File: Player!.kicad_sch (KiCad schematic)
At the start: 26 parts, among them J1 USB4085-GF-A_REVA4, J2 AVR-ISP-6, SW1 RotaryEncoder_Switch, SW2 SW_Push, SW3 SW_Push, SW4 SW_Push, SW5 SW_Push, SW6 Reset, SW7 Boot, U1 ATmega328P-P, Y1 Crystal

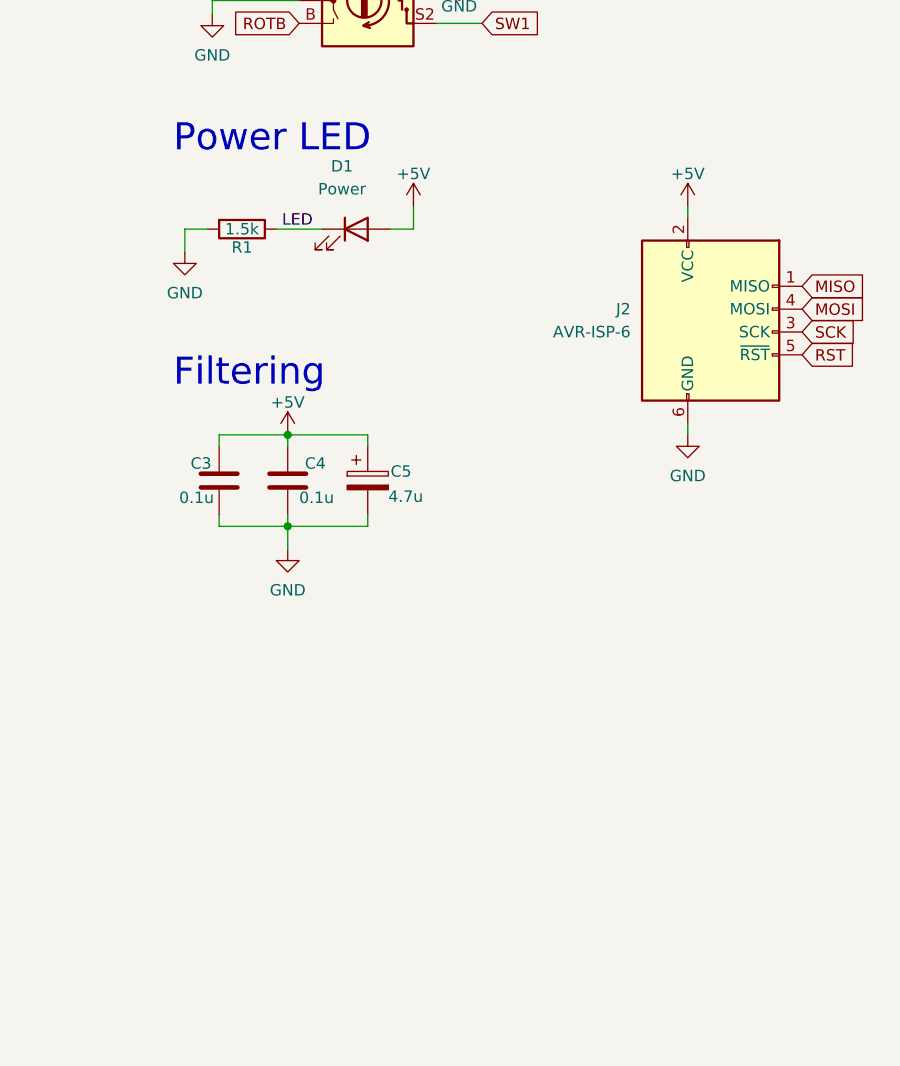
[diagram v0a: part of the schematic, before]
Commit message: Final PCB changes for v1.31
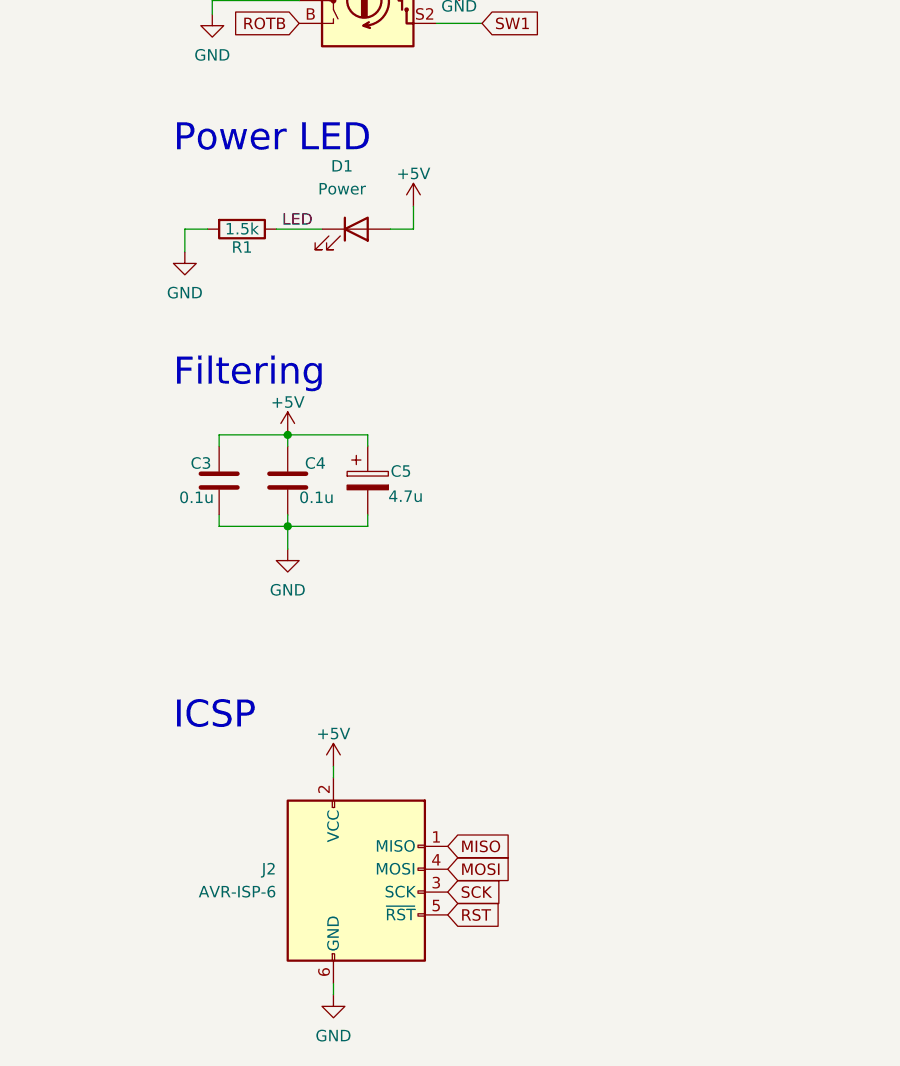
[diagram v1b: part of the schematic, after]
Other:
- note added: "ICSP"
- moved on the sheet: J2
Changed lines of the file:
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@@
     (stroke (width 0) (type default) (color 0 0 0 0))
   )
-  (wire (pts (xy 184.15 200.66) (xy 184.15 199.39))
+  (wire (pts (xy 144.78 262.89) (xy 144.78 261.62))
     (stroke (width 0) (type default) (color 0 0 0 0))
   )
@@
     (stroke (width 0) (type default) (color 0 0 0 0))
   )
-  (wire (pts (xy 184.15 175.26) (xy 184.15 176.53))
+  (wire (pts (xy 144.78 237.49) (xy 144.78 238.76))
     (stroke (width 0) (type default) (color 0 0 0 0))
   )
@@
   )
   (text "Filtering" (at 127 195.58 0)
+    (effects (font (size 3 3)) (justify left bottom))
+  )
+  (text "ICSP" (at 127 233.68 0)
     (effects (font (size 3 3)) (justify left bottom))
   )
@@
     )
   )
-  (global_label "SCK" (shape input) (at 196.85 189.23 0) (fields_autoplaced)
-    (effects (font (size 1.27 1.27)) (justify left))
-    (property "Intersheet References" "${INTERSHEET_REFS}" (id 0) (at 203.0126 189.1506 0)
+  (global_label "SCK" (shape input) (at 157.48 251.46 0) (fields_autoplaced)
+    (effects (font (size 1.27 1.27)) (justify left))
+    (property "Intersheet References" "${INTERSHEET_REFS}" (id 0) (at 163.6426 251.3806 0)
       (effects (font (size 1.27 1.27)) (justify left) hide)
     )
@@
     )
   )
-  (global_label "MISO" (shape input) (at 196.85 184.15 0) (fields_autoplaced)
-    (effects (font (size 1.27 1.27)) (justify left))
-    (property "Intersheet References" "${INTERSHEET_REFS}" (id 0) (at 203.8593 184.0706 0)
+  (global_label "MISO" (shape input) (at 157.48 246.38 0) (fields_autoplaced)
+    (effects (font (size 1.27 1.27)) (justify left))
+    (property "Intersheet References" "${INTERSHEET_REFS}" (id 0) (at 164.4893 246.3006 0)
       (effects (font (size 1.27 1.27)) (justify left) hide)
     )
@@
     )
   )
-  (global_label "MOSI" (shape input) (at 196.85 186.69 0) (fields_autoplaced)
-    (effects (font (size 1.27 1.27)) (justify left))
-    (property "Intersheet References" "${INTERSHEET_REFS}" (id 0) (at 203.8593 186.6106 0)
-      (effects (font (size 1.27 1.27)) (justify left) hide)
-    )
-  )
-  (global_label "RST" (shape input) (at 196.85 191.77 0) (fields_autoplaced)
-    (effects (font (size 1.27 1.27)) (justify left))
-    (property "Intersheet References" "${INTERSHEET_REFS}" (id 0) (at 202.7102 191.6906 0)
+  (global_label "MOSI" (shape input) (at 157.48 248.92 0) (fields_autoplaced)
+    (effects (font (size 1.27 1.27)) (justify left))
+    (property "Intersheet References" "${INTERSHEET_REFS}" (id 0) (at 164.4893 248.8406 0)
+      (effects (font (size 1.27 1.27)) (justify left) hide)
+    )
+  )
+  (global_label "RST" (shape input) (at 157.48 254 0) (fields_autoplaced)
+    (effects (font (size 1.27 1.27)) (justify left))
+    (property "Intersheet References" "${INTERSHEET_REFS}" (id 0) (at 163.3402 253.9206 0)
       (effects (font (size 1.27 1.27)) (justify left) hide)
     )
@@
     (pin "2")
   )
-  (symbol (lib_id "power:GND") (at 184.15 200.66 0) (unit 1)
+  (symbol (lib_id "power:GND") (at 144.78 262.89 0) (unit 1)
     (in_bom yes) (on_board yes) (fields_autoplaced)
-    (property "Reference" "#PWR0102" (id 0) (at 184.15 207.01 0)
-      (effects (font (size 1.27 1.27)) hide)
-    )
-    (property "Value" "GND" (id 1) (at 184.15 205.2225 0))
-    (property "Footprint" "" (id 2) (at 184.15 200.66 0)
-      (effects (font (size 1.27 1.27)) hide)
-    )
-    (property "Datasheet" "" (id 3) (at 184.15 200.66 0)
+    (property "Reference" "#PWR0102" (id 0) (at 144.78 269.24 0)
+      (effects (font (size 1.27 1.27)) hide)
+    )
+    (property "Value" "GND" (id 1) (at 144.78 267.4525 0))
+    (property "Footprint" "" (id 2) (at 144.78 262.89 0)
+      (effects (font (size 1.27 1.27)) hide)
+    )
+    (property "Datasheet" "" (id 3) (at 144.78 262.89 0)
       (effects (font (size 1.27 1.27)) hide)
     )
@@
     (pin "1")
   )
-  (symbol (lib_id "power:+5V") (at 184.15 175.26 0) (unit 1)
+  (symbol (lib_id "power:+5V") (at 144.78 237.49 0) (unit 1)
     (in_bom yes) (on_board yes) (fields_autoplaced)
-    (property "Reference" "#PWR0101" (id 0) (at 184.15 179.07 0)
-      (effects (font (size 1.27 1.27)) hide)
-    )
-    (property "Value" "+5V" (id 1) (at 184.15 171.6555 0))
-    (property "Footprint" "" (id 2) (at 184.15 175.26 0)
-      (effects (font (size 1.27 1.27)) hide)
-    )
-    (property "Datasheet" "" (id 3) (at 184.15 175.26 0)
+    (property "Reference" "#PWR0101" (id 0) (at 144.78 241.3 0)
+      (effects (font (size 1.27 1.27)) hide)
+    )
+    (property "Value" "+5V" (id 1) (at 144.78 233.8855 0))
+    (property "Footprint" "" (id 2) (at 144.78 237.49 0)
+      (effects (font (size 1.27 1.27)) hide)
+    )
+    (property "Datasheet" "" (id 3) (at 144.78 237.49 0)
       (effects (font (size 1.27 1.27)) hide)
     )
@@
     (pin "2")
   )
-  (symbol (lib_id "Connector:AVR-ISP-6") (at 186.69 189.23 0) (unit 1)
+  (symbol (lib_id "Connector:AVR-ISP-6") (at 147.32 251.46 0) (unit 1)
     (in_bom yes) (on_board yes) (fields_autoplaced)
-    (property "Reference" "J2" (id 0) (at 177.8 186.6899 0)
+    (property "Reference" "J2" (id 0) (at 138.43 248.9199 0)
       (effects (font (size 1.27 1.27)) (justify right))
     )
-    (property "Value" "AVR-ISP-6" (id 1) (at 177.8 189.2299 0)
+    (property "Value" "AVR-ISP-6" (id 1) (at 138.43 251.4599 0)
       (effects (font (size 1.27 1.27)) (justify right))
     )
-    (property "Footprint" "Keyboard Stuff:PinHeader_2x03_P2.54mm_Vertical" (id 2) (at 180.34 187.96 90)
-      (effects (font (size 1.27 1.27)) hide)
-    )
-    (property "Datasheet" " ~" (id 3) (at 154.305 203.2 0)
-      (effects (font (size 1.27 1.27)) hide)
-    )
+    (property "Footprint" "Keyboard Stuff:PinHeader_2x03_P2.54mm_Vertical" (id 2) (at 140.97 250.19 90)
+      (effects (font (size 1.27 1.27)) hide)
+    )
+    (property "Datasheet" " ~" (id 3) (at 114.935 265.43 0)
+      (effects (font (size 1.27 1.27)) hide)
+    )
